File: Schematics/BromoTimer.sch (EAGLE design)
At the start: 29 parts, among them IC1 PIC16F687, IC2 7805TV, K1 G2R2A, K2 G2R2A, Q1 BC548B, Q2 BC548B, Q3 BC548B, X1 AC_IN, X4 22-23-2041, X5 AC_OUT

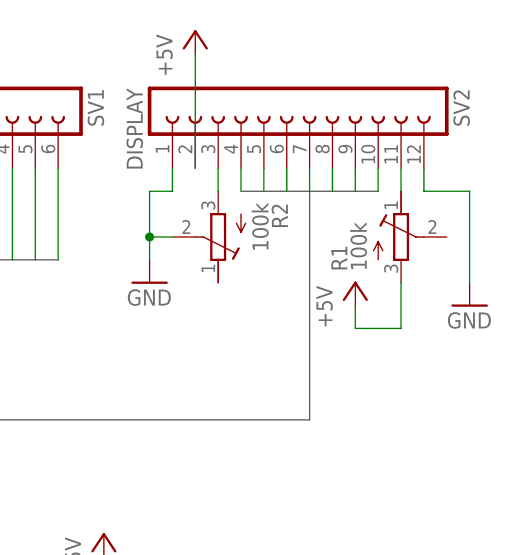
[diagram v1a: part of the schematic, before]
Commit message: Clean up R1
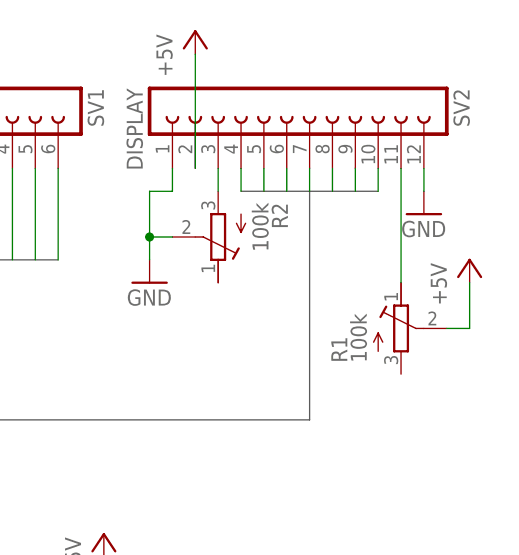
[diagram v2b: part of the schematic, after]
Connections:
- net +5V: now also R1.S; no longer R1.A
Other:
- moved on the sheet: R1
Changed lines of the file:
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@@
 <instance part="P+2" gate="1" x="124.46" y="134.62"/>
 <instance part="GND3" gate="1" x="193.04" y="142.24"/>
-<instance part="GND4" gate="1" x="228.6" y="139.7"/>
+<instance part="GND4" gate="1" x="223.52" y="149.86"/>
 <instance part="P+3" gate="1" x="198.12" y="170.18"/>
-<instance part="R1" gate="G$1" x="220.98" y="147.32"/>
+<instance part="R1" gate="G$1" x="220.98" y="137.16"/>
 <instance part="R2" gate="G$1" x="200.66" y="147.32" rot="R180"/>
-<instance part="P+4" gate="1" x="215.9" y="142.24"/>
+<instance part="P+4" gate="1" x="228.6" y="144.78"/>
 <instance part="Q1" gate="G$1" x="185.42" y="86.36"/>
 <instance part="Q2" gate="G$1" x="185.42" y="43.18"/>
@@
 </segment>
 <segment>
-<pinref part="P+4" gate="1" pin="+5V"/>
-<wire x1="215.9" y1="139.7" x2="215.9" y2="137.16" width="0.1524" layer="91"/>
-<pinref part="R1" gate="G$1" pin="A"/>
-<wire x1="215.9" y1="137.16" x2="220.98" y2="137.16" width="0.1524" layer="91"/>
-<wire x1="220.98" y1="137.16" x2="220.98" y2="142.24" width="0.1524" layer="91"/>
-</segment>
-<segment>
 <pinref part="SV3" gate="G$1" pin="2"/>
 <wire x1="129.54" y1="162.56" x2="129.54" y2="157.48" width="0.1524" layer="91"/>
@@
 <junction x="187.96" y="109.22"/>
 </segment>
+<segment>
+<pinref part="P+4" gate="1" pin="+5V"/>
+<wire x1="228.6" y1="142.24" x2="228.6" y2="137.16" width="0.1524" layer="91"/>
+<pinref part="R1" gate="G$1" pin="S"/>
+<wire x1="228.6" y1="137.16" x2="226.06" y2="137.16" width="0.1524" layer="91"/>
+</segment>
 </net>
 <net name="GND" class="0">
@@
 <pinref part="GND4" gate="1" pin="GND"/>
 <pinref part="SV2" gate="G$1" pin="12"/>
-<wire x1="228.6" y1="142.24" x2="228.6" y2="152.4" width="0.1524" layer="91"/>
-<wire x1="228.6" y1="152.4" x2="223.52" y2="152.4" width="0.1524" layer="91"/>
 <wire x1="223.52" y1="152.4" x2="223.52" y2="154.94" width="0.1524" layer="91"/>
 </segment>
@@
 <segment>
 <pinref part="SV2" gate="G$1" pin="11"/>
-<wire x1="220.98" y1="154.94" x2="220.98" y2="152.4" width="0.1524" layer="91"/>
+<wire x1="220.98" y1="154.94" x2="220.98" y2="142.24" width="0.1524" layer="91"/>
 <pinref part="R1" gate="G$1" pin="E"/>
 </segment>
